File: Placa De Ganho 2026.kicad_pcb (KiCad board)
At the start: 2 copper layers, 40 parts, among them J1 Conn_Output, J2 Conn_01x01_Pin, J3 Conn_Sensores, J4 Conn_Alimentacao, U1 AD625JNZ, U2 AD625JNZ, U3 AD744JNZ, U4 AD744JNZ

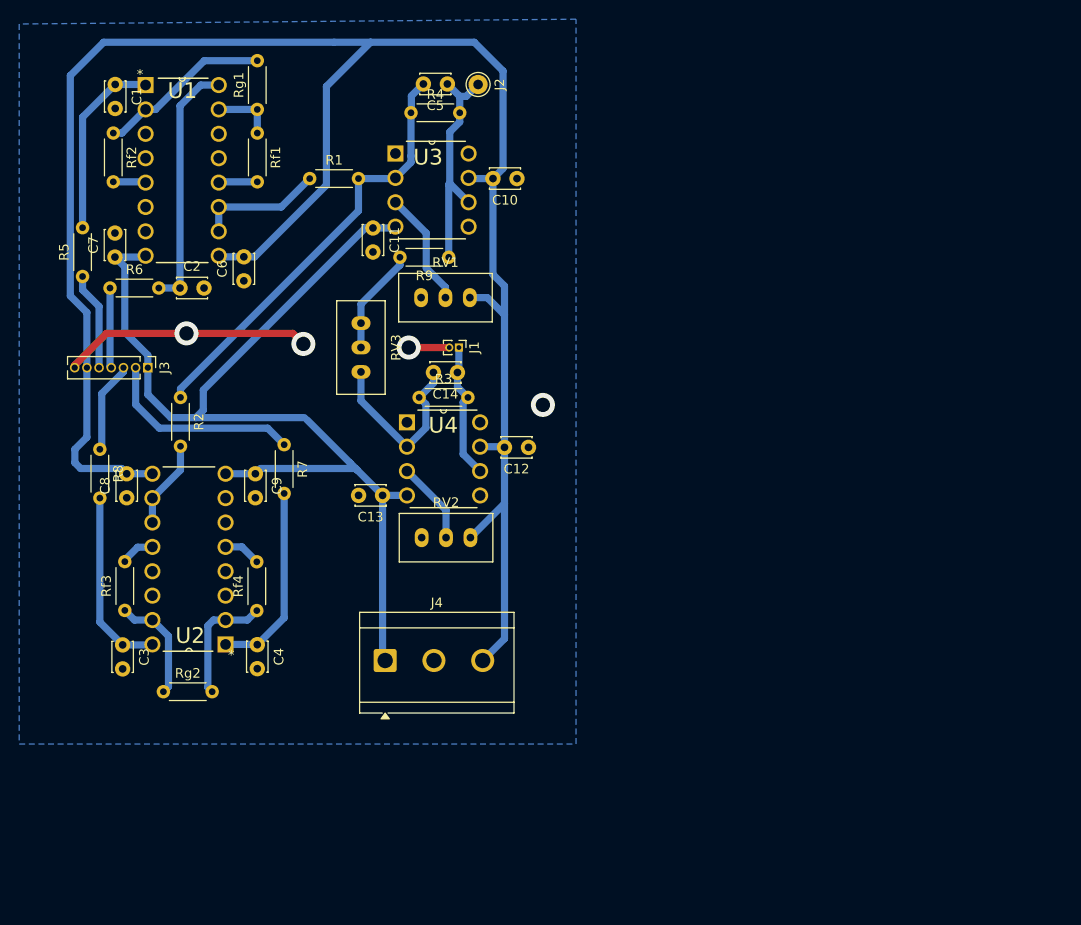
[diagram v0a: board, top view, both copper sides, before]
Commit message: 11_07_2026
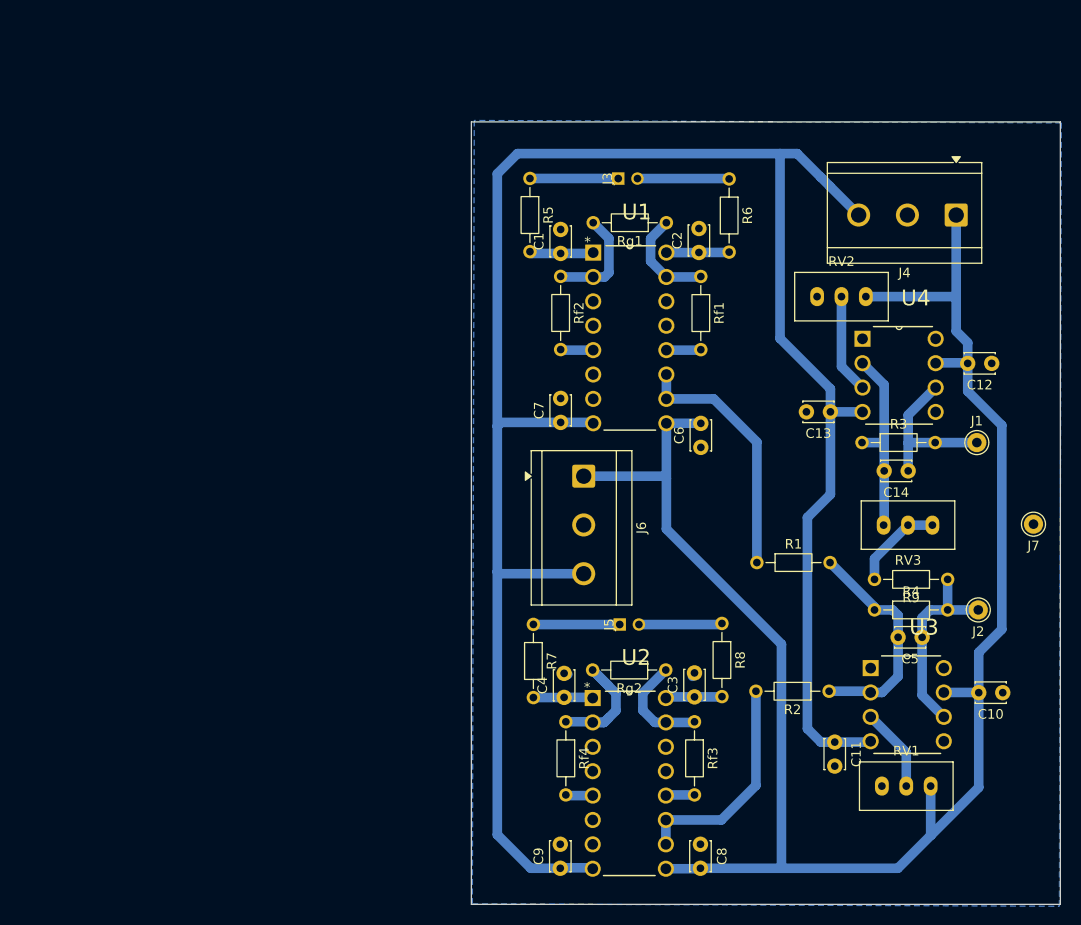
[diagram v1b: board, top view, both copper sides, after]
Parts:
- added J5: Conn_Wheatstone_02, Cangaco:CANGACO_PinHeader_1x02_0.8mm, F.Cu at (84.7, 86.0)
- added J6: Conn_Wheatstone_Alim, TerminalBlock_CUI:TerminalBlock_CUI_TB007-508-03_1x03_P5.08mm_Horizontal, F.Cu at (80.4, 70.6)
- added J7: Conn_Terra_Out, Connector_Pin:Pin_D1.0mm_L10.0mm, F.Cu at (127.2, 75.6)
- J1: value Conn_Output -> Conn_Estagio_3_Out; footprint Connector_PinHeader_1.00mm:PinHeader_1x02_P1.00mm_Vertical -> Connector_Pin:Pin_D1.0mm_L10.0mm
- J2: value Conn_01x01_Pin -> Conn_Estagio_2_Out
- J3: value Conn_Sensores -> Conn_Wheatstone01; footprint Connector_PinHeader_1.27mm:PinHeader_1x07_P1.27mm_Vertical -> Cangaco:CANGACO_PinHeader_1x02_0.8mm
- R1, R2, R3, R4, R5, R6, R7, R8, R9, Rf1, Rf2, Rf3, Rf4, Rg1, Rg2: footprint Resistor_THT:R_Axial_DIN0204_L3.6mm_D1.6mm_P5.08mm_Horizontal -> Cangaco:CANGACO_Resistor_0.8mm
- RV1, RV2, RV3: footprint Cangaço:SPACE-Potentiometer_Bourns_3296W_Vertical -> Cangaco:SPACE-Potentiometer_Bourns_3296W_Vertical
- moved C5 75.9 mm to (115.7, 87.4)
- moved J2 75.6 mm to (121.5, 84.5), turned to 0 degrees
- moved J4 75.4 mm to (119.2, 43.4), turned to 180 degrees
- moved R2 74.2 mm to (106.0, 93.0), turned to 180 degrees
- moved C10 73.7 mm to (124.0, 93.2)
- moved U3 73.0 mm to (117.9, 98.2)
- moved C11 72.0 mm to (106.5, 98.3)
- moved R4 70.8 mm to (110.7, 84.5)
- moved RV1 69.9 mm to (116.5, 102.9)
- moved C8 69.8 mm to (92.6, 108.9), turned to -90 degrees
- moved U2 67.5 mm to (89.0, 111.5), turned to 0 degrees
- moved R8 67.3 mm to (94.8, 85.9)
- moved R6 65.5 mm to (95.5, 39.6), turned to -90 degrees
- moved R9 61.9 mm to (118.3, 81.3)
- moved R1 61.4 mm to (98.4, 79.6)
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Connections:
- J3 pad 1: VSS -> Net-(J3-Pin_1)
- J3 pad 2: Net-(J3-Pin_3) -> Net-(J3-Pin_2)
- J4 pad 1: VSS -> VDD
- J4 pad 3: VDD -> VSS
- R7 pad 1: Net-(J3-Pin_3) -> Net-(J5-Pin_1)
- R8 pad 1: Net-(J3-Pin_4) -> Net-(J5-Pin_2)
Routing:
- net VSS: track 111.5 -> 214.0 mm
- net GND: track 30.6 -> 0.59 mm, vias 4 -> 0
- net VDD: track 207.1 -> 183.4 mm
- net Net-(U3--IN): track 45.3 -> 23.8 mm
- net Net-(J3-Pin_3): track 21.0 -> 0.00 mm
- net Net-(U1--IN): track 26.5 -> 6.56 mm
- net Net-(U2-SENSE): track 9.16 -> 23.2 mm
- net Net-(U2-+IN): track 20.2 -> 6.22 mm
- net Net-(U2--IN): track 19.4 -> 6.10 mm
- net Net-(U1-SENSE): track 13.2 -> 26.4 mm
- net Net-(U1-+IN): track 19.6 -> 6.71 mm
- net Net-(J3-Pin_4): track 9.52 -> 0.00 mm
- net Net-(J5-Pin_1): track 0.00 -> 8.99 mm
- net Net-(J5-Pin_2): track 0.00 -> 8.70 mm
- net Net-(U1-+GAIN_SEN): track 18.1 -> 11.1 mm
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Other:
- board outline added: 61.4 x 81.5 mm
